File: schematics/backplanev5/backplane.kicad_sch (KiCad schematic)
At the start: 28 parts, among them J12 Conn_01x02, J13 Conn_01x02, J14 Conn_01x02

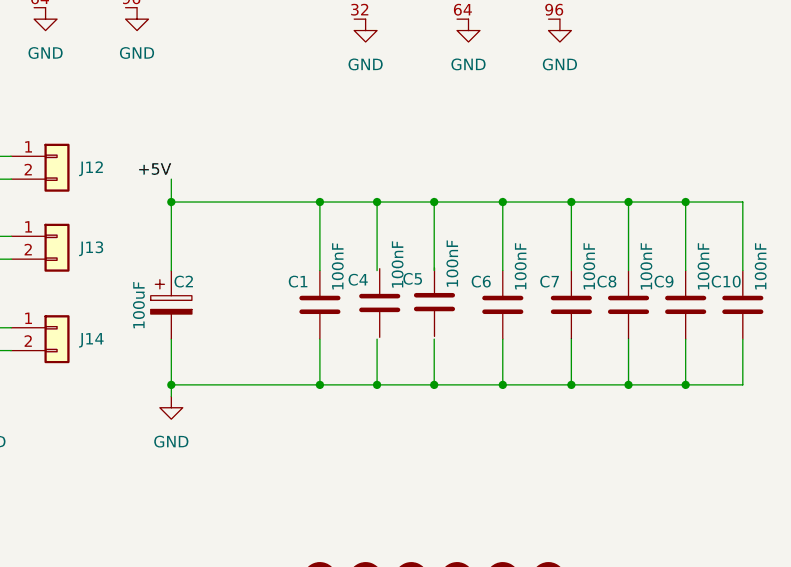
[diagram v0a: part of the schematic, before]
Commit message: Terminado o DRC
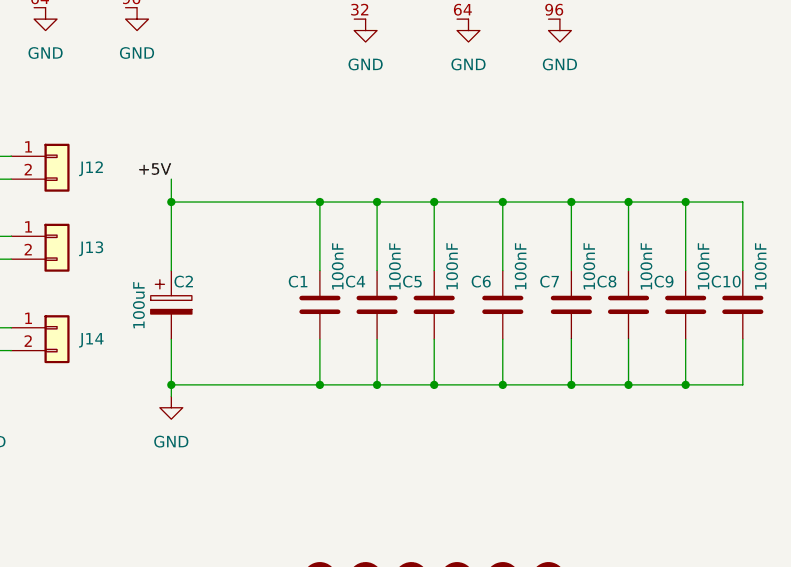
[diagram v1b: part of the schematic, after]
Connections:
- net +5V: now also C4.1, C5.1
- net GND: now also C4.2, C5.2
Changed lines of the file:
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@@
 	(symbol
 		(lib_id "Device:C")
-		(at 246.41 127.9638 0)
+		(at 246.38 128.27 0)
 		(unit 1)
 		(exclude_from_sim no)
@@
 		(dnp no)
 		(property "Reference" "C5"
-			(at 242.854 125.4238 0)
+			(at 242.824 125.73 0)
 			(effects
 				(font
@@
 		)
 		(property "Value" "100nF"
-			(at 248.442 126.4398 90)
+			(at 248.412 126.746 90)
 			(effects
 				(font
@@
 		)
 		(property "Footprint" "Capacitor_THT:C_Disc_D4.3mm_W1.9mm_P5.00mm"
-			(at 247.3752 131.7738 0)
+			(at 247.3452 132.08 0)
 			(effects
 				(font
@@
 		)
 		(property "Datasheet" "~"
-			(at 246.41 127.9638 0)
+			(at 246.38 128.27 0)
 			(effects
 				(font
@@
 		)
 		(property "Description" "Unpolarized capacitor"
-			(at 246.41 127.9638 0)
+			(at 246.38 128.27 0)
 			(effects
 				(font
@@
 	(symbol
 		(lib_id "Device:C")
-		(at 240.3251 128.0619 0)
+		(at 240.03 128.27 0)
 		(unit 1)
 		(exclude_from_sim no)
@@
 		(dnp no)
 		(property "Reference" "C4"
-			(at 236.7691 125.5219 0)
+			(at 236.474 125.73 0)
 			(effects
 				(font
@@
 		)
 		(property "Value" "100nF"
-			(at 242.3571 126.5379 90)
+			(at 242.062 126.746 90)
 			(effects
 				(font
@@
 		)
 		(property "Footprint" "Capacitor_THT:C_Disc_D4.3mm_W1.9mm_P5.00mm"
-			(at 241.2903 131.8719 0)
+			(at 240.9952 132.08 0)
 			(effects
 				(font
@@
 		)
 		(property "Datasheet" "~"
-			(at 240.3251 128.0619 0)
+			(at 240.03 128.27 0)
 			(effects
 				(font
@@
 		)
 		(property "Description" "Unpolarized capacitor"
-			(at 240.3251 128.0619 0)
-			(effects
-				(font
+			(at 240.03 128.27 0)
+			(effects
+				(font
